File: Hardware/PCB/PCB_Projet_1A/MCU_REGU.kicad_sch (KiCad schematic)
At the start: 18 parts, among them J10 Conn_01x02, J11 BU33SD5WG-TR, J12 R-78B5.0-2.0, U2 STM32L552CCTx

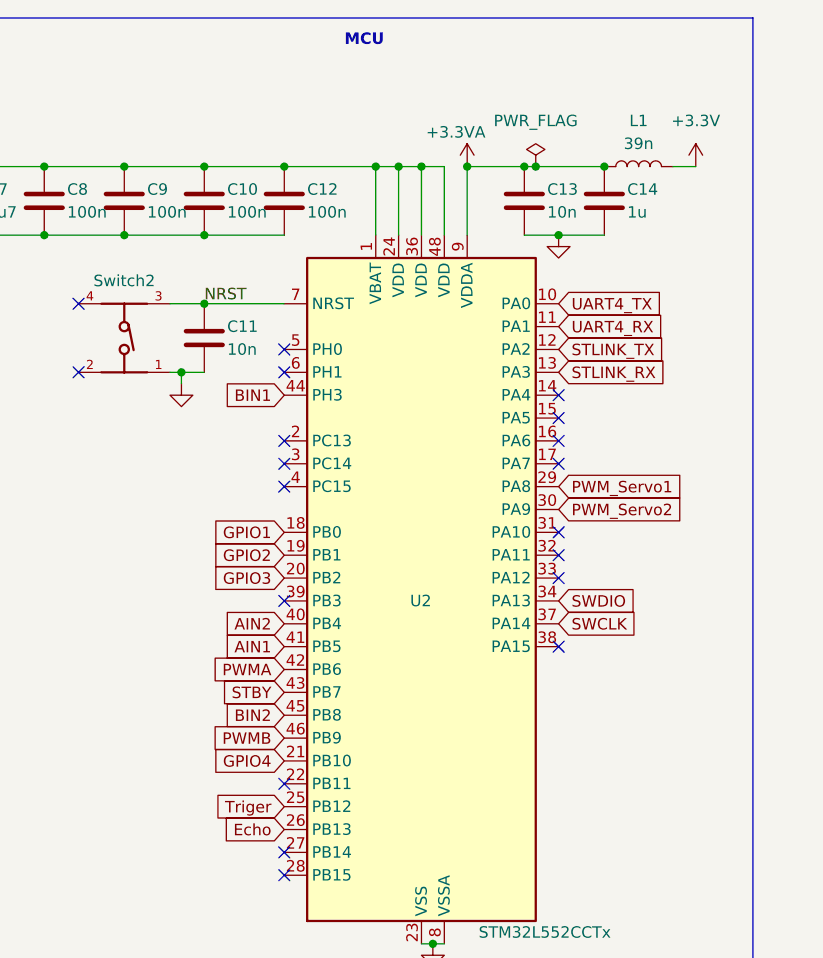
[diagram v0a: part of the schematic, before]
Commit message: modif pcb
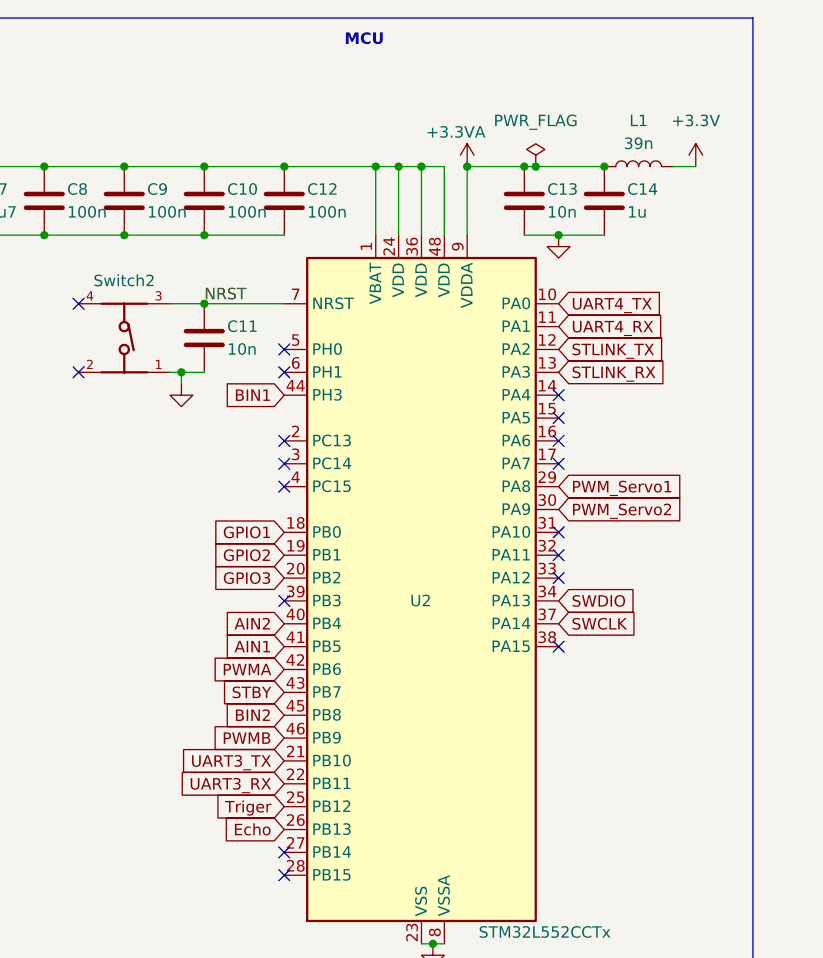
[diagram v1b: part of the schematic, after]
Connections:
- net UART3_RX: now reaches U2.22 (PB11)
- net GPIO4 renamed UART3_TX
- no-connect marks 19 -> 18
